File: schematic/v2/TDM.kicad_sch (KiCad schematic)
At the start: 21 parts, among them J18 LCD_display, U6 BME280, U9 NUCLEO-F446RE

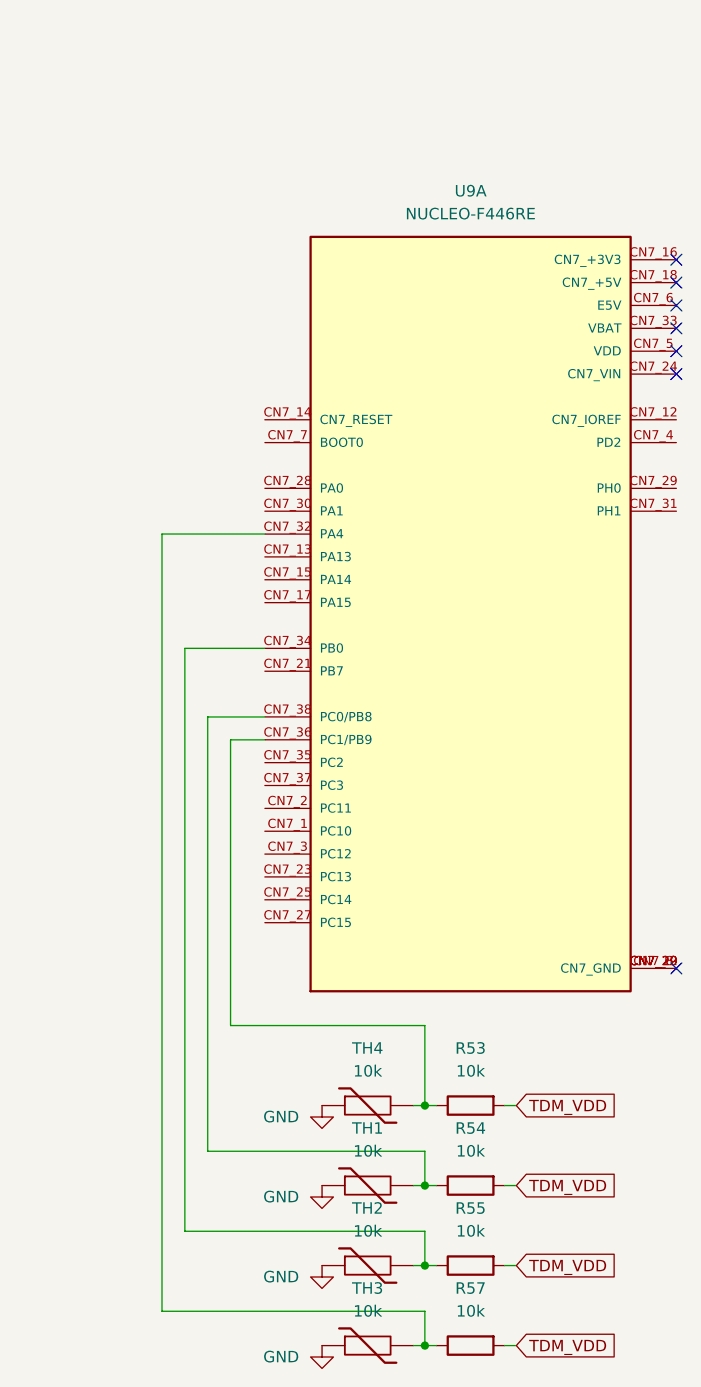
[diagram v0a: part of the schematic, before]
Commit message: hmmm figuring out filter module right now
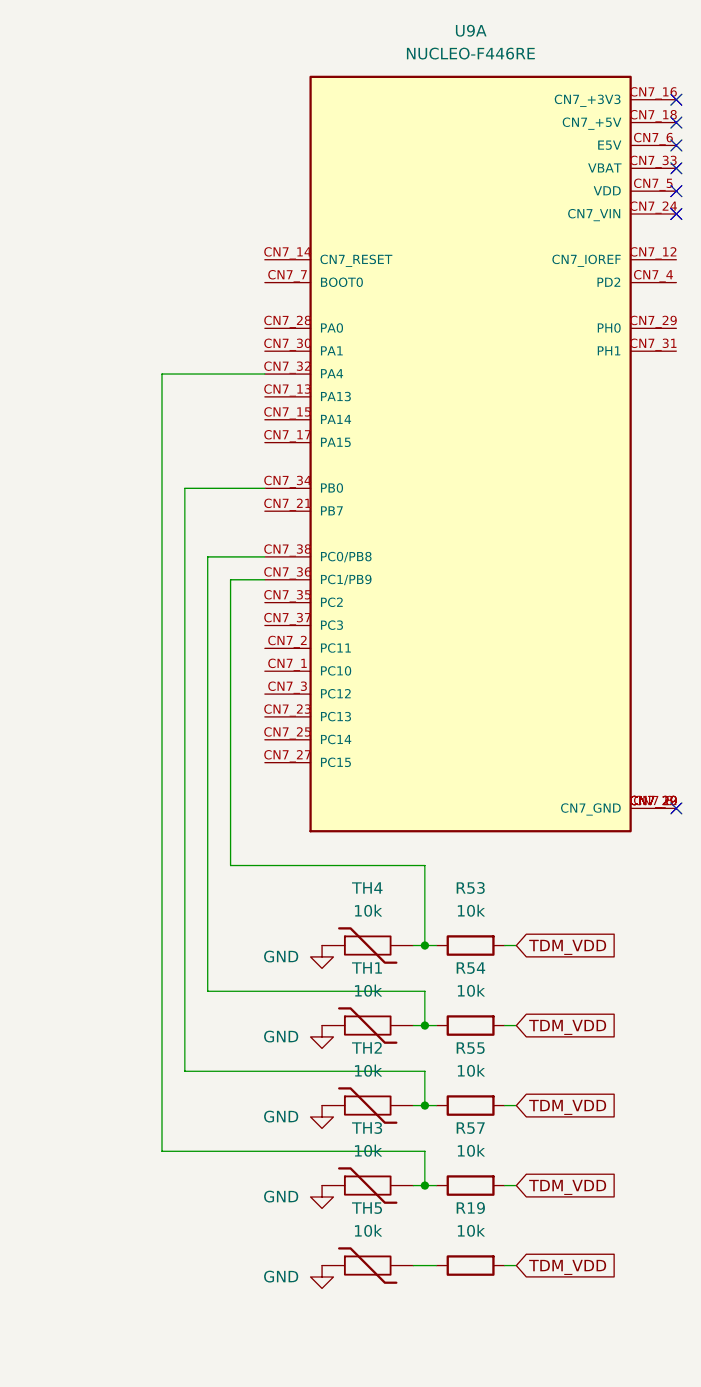
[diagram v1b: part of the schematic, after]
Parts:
- added R19: 10k, Resistor_SMD:R_0805_2012Metric_Pad1.20x1.40mm_HandSolder, symbol Device:R
- added TH5: 10k, Package_TO_SOT_THT:Heraeus_TO-92-2, symbol Device:Thermistor
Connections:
- net 5V_TDM: now also R19.2
- net GND: now also TH5.1
- new net: R19.1, TH5.2
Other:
- moved on the sheet: R53, R54, R55, R57, TH1, TH2, TH3, TH4, U9A
